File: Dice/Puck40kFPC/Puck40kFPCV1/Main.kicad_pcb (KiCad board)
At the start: 2 copper layers, 35.6 x 25.9 mm, 9 parts, among them J5 Conn_01x06

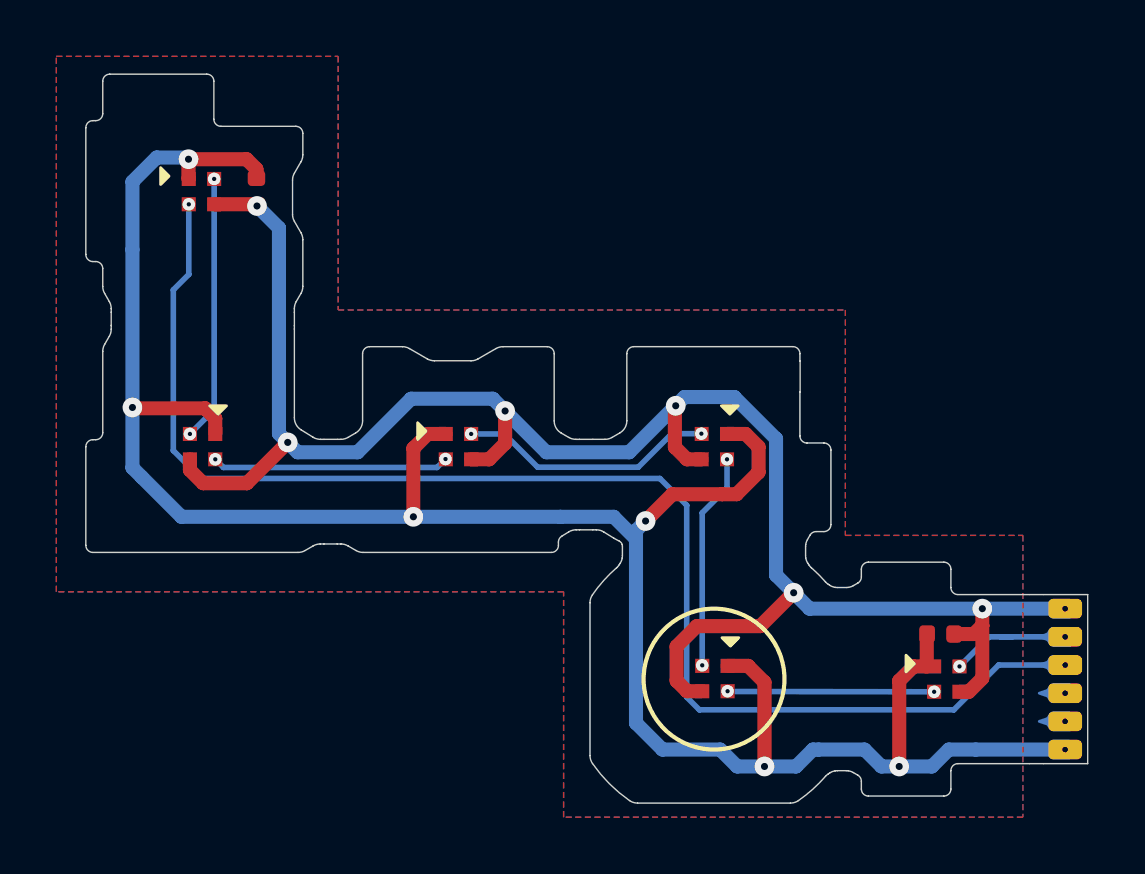
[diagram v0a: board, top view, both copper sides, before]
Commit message: more board file updates
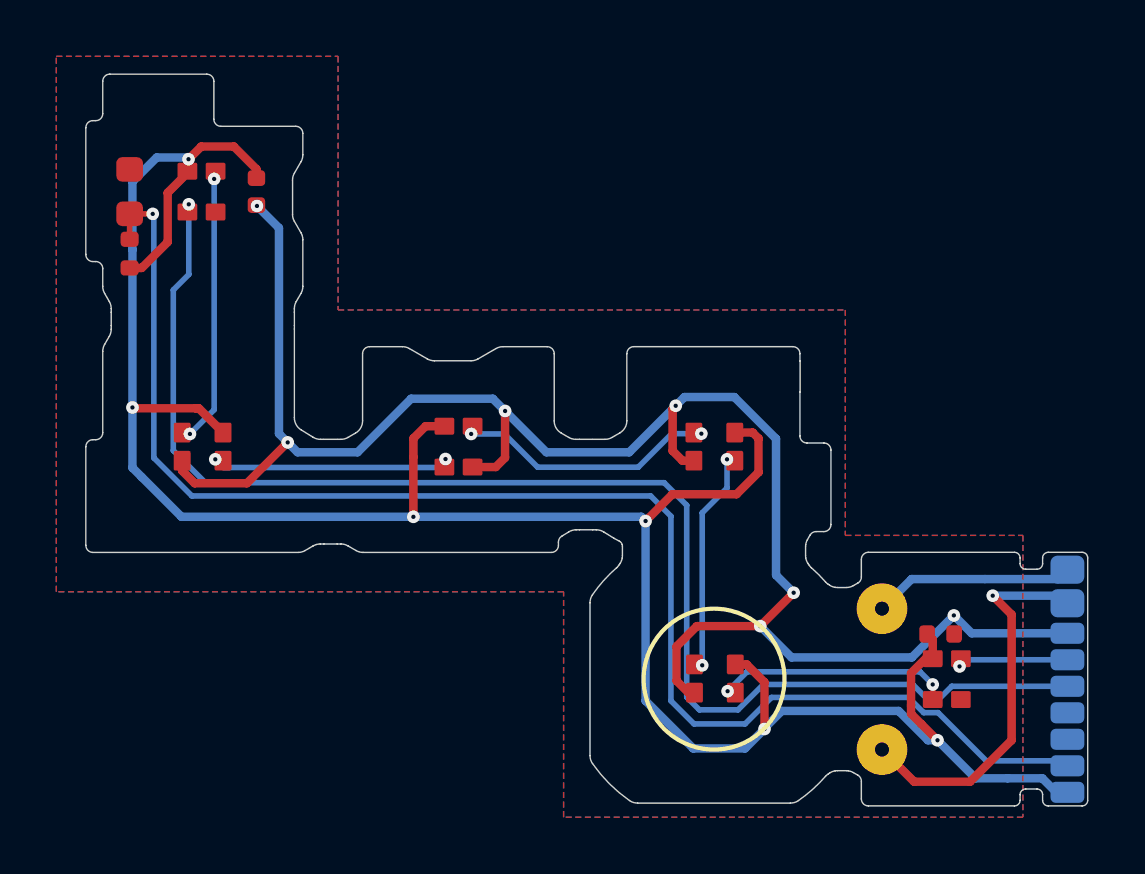
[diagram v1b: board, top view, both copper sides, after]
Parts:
- added P5: COILA, Pixels-dice:TestPoint_THTPad_D1.5mm_Drill0.7mm_nosilk, F.Cu at (158.3, 109.6)
- added P6: COILB, Pixels-dice:TestPoint_THTPad_D1.5mm_Drill0.7mm_nosilk, F.Cu at (158.3, 114.6)
- added Q1: ZSPT-Z1608C-06F-Z4, Diode_SMD:D_0603_1608Metric, F.Cu at (131.6, 94.8)
- added R5: 10k 1%, Resistor_SMD:R_0402_1005Metric, F.Cu at (131.6, 97.0)
- D1, D2, D3, D4, D5, D6: value SK6805-EC14 -> TX1812MJA5; footprint Pixels-dice:SK6805-EC14 -> Pixels-dice:TX1812MWCA5-F01
- J5: value Conn_01x06 -> Conn_01x09; footprint Pixels-dice:LED_CONNECTOR_6_FPC -> Pixels-dice:LED_CONNECTOR_9; moved to B.Cu
- moved J5 1.51 mm to (164.9, 110.7)
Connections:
- D1 pad 1: VDC -> Net-(D1-DOUT)
- D1 pad 2: Net-(D1-DOUT) -> GND
- D1 pad 3: GND -> /LED_DATA
- D1 pad 4: /LED_DATA -> VDC
- D2 pad 1: VDC -> Net-(D2-DOUT)
- D2 pad 2: Net-(D2-DOUT) -> GND
- D2 pad 3: GND -> Net-(D1-DOUT)
- D2 pad 4: Net-(D1-DOUT) -> VDC
- D3 pad 1: VDC -> Net-(D3-DOUT)
- D3 pad 2: Net-(D3-DOUT) -> GND
- D3 pad 3: GND -> Net-(D2-DOUT)
- D3 pad 4: Net-(D2-DOUT) -> VDC
- D4 pad 1: VDC -> Net-(D4-DOUT)
- D4 pad 2: Net-(D4-DOUT) -> GND
- D4 pad 3: GND -> Net-(D3-DOUT)
- D4 pad 4: Net-(D3-DOUT) -> VDC
- D5 pad 1: VDC -> Net-(D5-DOUT)
- D5 pad 2: Net-(D5-DOUT) -> GND
- D5 pad 3: GND -> Net-(D4-DOUT)
- D5 pad 4: Net-(D4-DOUT) -> VDC
- D6 pad 1: VDC -> /LED_RETURN
- D6 pad 2: /LED_RETURN -> GND
- D6 pad 3: GND -> Net-(D5-DOUT)
- D6 pad 4: Net-(D5-DOUT) -> VDC
- J5 pad 1: GND -> /COILA
- J5 pad 2: /LED_DATA -> /COILB
- J5 pad 3: /LED_RETURN -> GND
- J5 pad 4: unconnected-(J5-Pin_4-Pad4)_1 -> /LED_DATA
- J5 pad 5: +BATT -> /LED_RETURN
- J5 pad 6: VDC -> VDD
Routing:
- net /OPT_A2D: track 0.00 -> 52.0 mm, vias 0 -> 1
- net /COILB: track 0.00 -> 13.8 mm, vias 0 -> 1
- net /COILA: track 0.00 -> 7.15 mm
- net GND: track 67.8 -> 64.7 mm, vias 6 -> 7
- net VDC: track 83.0 -> 85.3 mm
- net Net-(D1-DOUT): track 7.34 -> 8.29 mm
- net /LED_RETURN: track 48.7 -> 49.3 mm
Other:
- board size 35.6 x 25.9 mm -> 35.6 x 26 mm
